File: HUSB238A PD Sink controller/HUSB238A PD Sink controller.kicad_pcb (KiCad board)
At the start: 2 copper layers, 38.1 x 45.7 mm, 74 parts, among them J2 VSET, J4 ISET, J6 I2C, U2 HUSB238A-xxxxx-QN16R

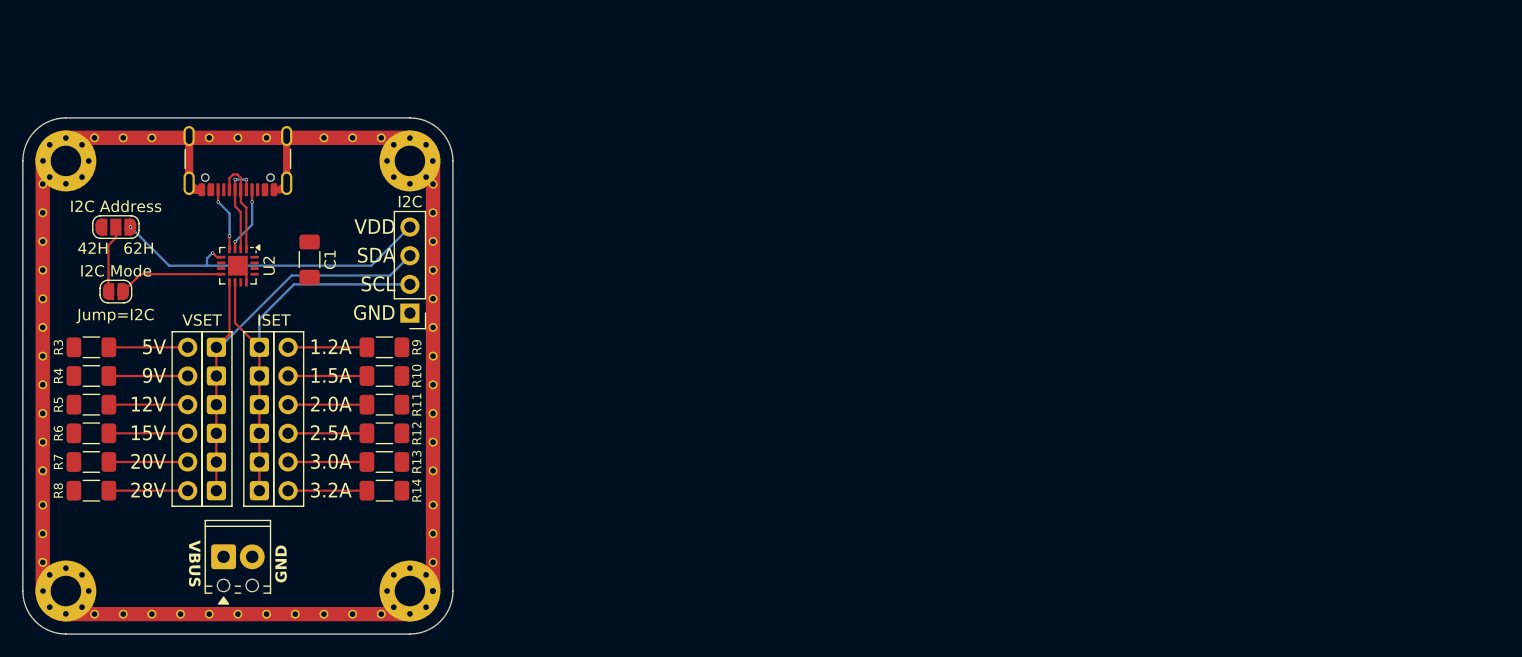
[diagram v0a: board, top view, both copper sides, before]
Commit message: R2.3
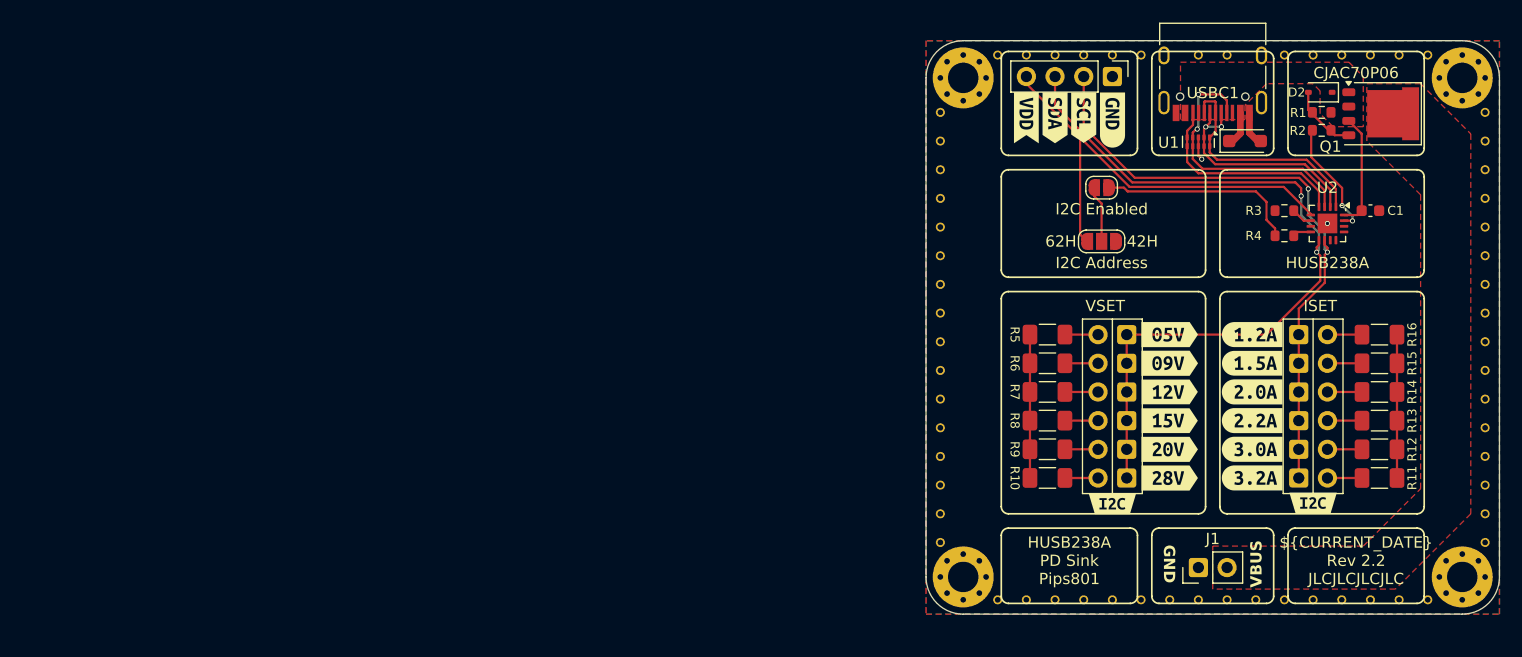
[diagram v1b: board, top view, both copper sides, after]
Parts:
- removed the ? at (94.0, 112.5)
- removed the ? at (84.3, 97.3)
- removed the ? at (88.9, 70.3)
- removed the ? at (118.9, 92.2)
- removed the ? at (118.9, 102.9)
- removed the ? at (99.1, 70.3)
- removed the ? at (84.3, 99.8)
- removed the ? at (118.9, 74.4)
- removed the ? at (84.3, 82.1)
- removed the ? at (84.3, 74.4)
- removed the ? at (114.3, 70.3)
- removed the ? at (118.9, 105.4)
- removed the ? at (118.9, 99.8)
- removed the ? at (84.3, 79.5)
- removed the ? at (118.9, 94.8)
- removed the ? at (84.3, 94.8)
- removed the ? at (84.3, 77.0)
- removed the ? at (106.7, 112.5)
- removed the ? at (91.4, 70.3)
- removed the ? at (84.3, 84.6)
- removed the ? at (118.9, 84.6)
- removed the ? at (104.1, 112.5)
- removed the ? at (118.9, 82.1)
- removed the ? at (84.3, 102.9)
- removed the ? at (114.3, 112.5)
- removed the ? at (118.9, 97.3)
- removed the ? at (84.3, 87.1)
- removed the ? at (104.1, 70.3)
- removed the ? at (111.8, 70.3)
- removed the ? at (84.3, 108.0)
- removed the ? at (99.1, 112.5)
- removed the ? at (96.5, 112.5)
- removed the ? at (84.3, 92.2)
- removed the ? at (101.6, 70.3)
- removed the ? at (118.9, 110.5)
- removed the ? at (94.0, 70.3)
- removed the ? at (118.9, 79.5)
- removed the ? at (118.9, 89.7)
- removed the ? at (118.9, 87.1)
- removed the ? at (88.9, 112.5)
- removed the ? at (91.4, 112.5)
- removed the ? at (84.3, 105.4)
- removed the ? at (109.2, 70.3)
- removed the ? at (101.6, 112.5)
- removed the ? at (84.3, 89.7)
- removed the ? at (109.2, 112.5)
- removed the ? at (118.9, 108.0)
- removed the ? at (118.9, 77.0)
- removed the ? at (111.8, 112.5)
- removed J6: I2C, Connector_PinHeader_2.54mm:PinHeader_1x04_P2.54mm_Vertical
- removed the REF** at (86.4, 110.5)
- removed the REF** at (86.4, 72.4)
- removed the REF** at (116.8, 72.4)
- removed the REF** at (116.8, 110.5)
- added ?: , , F.Cu at (163.8, 78.2)
- added ?: , , F.Cu at (171.4, 111.3)
- added ?: , , F.Cu at (163.8, 83.3)
- added ?: , , F.Cu at (163.8, 70.6)
- added ?: , , F.Cu at (212.1, 75.7)
- added ?: , , F.Cu at (163.8, 73.2)
- added ?: , , F.Cu at (163.8, 106.2)
- added ?: , , F.Cu at (174.0, 63.0)
- added ?: , , F.Cu at (186.7, 111.3)
- added ?: , , F.Cu at (179.1, 63.0)
- added ?: , , F.Cu at (212.1, 93.5)
- added ?: , , F.Cu at (189.2, 63.0)
- added ?: , , F.Cu at (212.1, 106.2)
- added ?: , , F.Cu at (212.1, 90.9)
- added ?: , , F.Cu at (212.1, 85.9)
- added ?: , , F.Cu at (212.1, 68.1)
- added ?: , , F.Cu at (181.6, 111.3)
- added ?: , , F.Cu at (212.1, 83.3)
- added ?: , , F.Cu at (212.1, 70.6)
- added ?: , , F.Cu at (212.1, 88.4)
- added ?: , , F.Cu at (212.1, 73.2)
- added ?: , , F.Cu at (212.1, 103.6)
- added ?: , , F.Cu at (199.4, 63.0)
- added ?: , , F.Cu at (176.5, 63.0)
- added ?: , , F.Cu at (204.5, 63.0)
- added ?: , , F.Cu at (194.3, 63.0)
- added ?: , , F.Cu at (168.9, 111.3)
- added ?: , , F.Cu at (176.5, 111.3)
- added ?: , , F.Cu at (171.4, 63.0)
- added ?: , , F.Cu at (174.0, 111.3)
- added ?: , , F.Cu at (163.8, 85.9)
- added ?: , , F.Cu at (163.8, 88.4)
- added ?: , , F.Cu at (207.0, 63.0)
- added ?: , , F.Cu at (163.8, 90.9)
- added ?: , , F.Cu at (184.2, 111.3)
- added ?: , , F.Cu at (181.6, 63.0)
- added ?: , , F.Cu at (191.8, 111.3)
- added ?: , , F.Cu at (163.8, 101.1)
- added ?: , , F.Cu at (212.1, 96.0)
- added ?: , , F.Cu at (207.0, 111.3)
- added ?: , , F.Cu at (163.8, 103.6)
- added ?: , , F.Cu at (212.1, 98.6)
- added ?: , , F.Cu at (212.1, 78.2)
- added ?: , , F.Cu at (189.2, 111.3)
- added ?: , , F.Cu at (201.9, 111.3)
- added ?: , , F.Cu at (194.3, 111.3)
- added ?: , , F.Cu at (196.8, 63.0)
- added ?: , , F.Cu at (168.9, 63.0)
- added ?: , , F.Cu at (163.8, 80.8)
- added ?: , , F.Cu at (163.8, 68.1)
- added ?: , , F.Cu at (212.1, 80.8)
- added ?: , , F.Cu at (179.1, 111.3)
- added ?: , , F.Cu at (186.7, 63.0)
- added ?: , , F.Cu at (163.8, 75.7)
- added ?: , , F.Cu at (199.4, 111.3)
- added ?: , , F.Cu at (201.9, 63.0)
- added ?: , , F.Cu at (163.8, 96.0)
- added ?: , , F.Cu at (204.5, 111.3)
- added ?: , , F.Cu at (163.8, 98.6)
- added ?: , , F.Cu at (196.8, 111.3)
- added ?: , , F.Cu at (212.1, 101.1)
- added ?: , , F.Cu at (163.8, 93.5)
- added D1: ≥48V TVS Clamp, Diode_SMD:D_SOD-123F, F.Cu at (190.8, 70.6)
- added D2: 15V, Diode_SMD:D_SOD-323, F.Cu at (197.5, 66.3)
- added G***: LOGO, LOGO, B.Cu at (188.0, 87.1)
- added J3: I2C, Connector_PinHeader_2.54mm:PinHeader_1x04_P2.54mm_Vertical, F.Cu at (179.1, 64.9)
- added Q1: CJAC70P06, Package_DFN_QFN:PQFN-8-EP_6x5mm_P1.27mm_Generic, F.Cu at (202.7, 68.2)
- added R1: 100kΩ, Resistor_SMD:R_0603_1608Metric, F.Cu at (197.6, 68.1)
- added R2: 20kΩ, Resistor_SMD:R_0603_1608Metric, F.Cu at (197.6, 69.7)
- added R3: 900kΩ, Resistor_SMD:R_0603_1608Metric, F.Cu at (194.3, 76.8)
- added R4: 900kΩ, Resistor_SMD:R_0603_1608Metric, F.Cu at (194.3, 79.0)
- added REF**: MountingHole_2.7mm_M2.5_Pad_Via, MountingHole:MountingHole_2.7mm_M2.5_Pad_Via, F.Cu at (165.9, 65.0)
- added REF**: MountingHole_2.7mm_M2.5_Pad_Via, MountingHole:MountingHole_2.7mm_M2.5_Pad_Via, F.Cu at (210.1, 65.0)
- added REF**: MountingHole_2.7mm_M2.5_Pad_Via, MountingHole:MountingHole_2.7mm_M2.5_Pad_Via, F.Cu at (210.1, 109.2)
- added REF**: MountingHole_2.7mm_M2.5_Pad_Via, MountingHole:MountingHole_2.7mm_M2.5_Pad_Via, F.Cu at (165.9, 109.2)
- added U1: TPD4E05U06DQA, Package_SON:USON-10_2.5x1.0mm_P0.5mm, F.Cu at (186.7, 70.7)
- added kibuzzard-6951C990: G***, kibuzzard-6951C990, F.Cu at (179.1, 102.8)
- added kibuzzard-6951C990: G***, kibuzzard-6951C990, F.Cu at (196.8, 102.7)
- added kibuzzard-6951CA75: G***, kibuzzard-6951CA75, F.Cu at (184.2, 92.9)
- added kibuzzard-6951CAED: G***, kibuzzard-6951CAED, F.Cu at (184.2, 95.4)
- added kibuzzard-6951CAFD: G***, kibuzzard-6951CAFD, F.Cu at (184.2, 97.9)
- added kibuzzard-6951CB2B: G***, kibuzzard-6951CB2B, F.Cu at (184.2, 100.5)
- added kibuzzard-6951CB42: G***, kibuzzard-6951CB42, F.Cu at (191.5, 87.8)
- added kibuzzard-6951CB4D: G***, kibuzzard-6951CB4D, F.Cu at (191.5, 90.3)
- added kibuzzard-6951CB7E: G***, kibuzzard-6951CB7E, F.Cu at (191.5, 92.9)
- added kibuzzard-6951CEE5: G***, kibuzzard-6951CEE5, F.Cu at (191.5, 95.4)
- added kibuzzard-6951CF0B: G***, kibuzzard-6951CF0B, F.Cu at (191.5, 97.9)
- added kibuzzard-6951CF1D: G***, kibuzzard-6951CF1D, F.Cu at (191.5, 100.5)
- added kibuzzard-6951CF39: G***, kibuzzard-6951CF39, F.Cu at (184.2, 87.8)
- added kibuzzard-6951CF4B: G***, kibuzzard-6951CF4B, F.Cu at (184.2, 90.3)
- added kibuzzard-6951D5A7: G***, kibuzzard-6951D5A7, F.Cu at (179.1, 68.8)
- added kibuzzard-6951D5B1: G***, kibuzzard-6951D5B1, F.Cu at (176.5, 68.6)
- added kibuzzard-6951D5BC: G***, kibuzzard-6951D5BC, F.Cu at (174.0, 68.6)
- added kibuzzard-6951D5C7: G***, kibuzzard-6951D5C7, F.Cu at (171.4, 68.6)
- C1: footprint Capacitor_SMD:C_1206_3216Metric_Pad1.33x1.80mm_HandSolder -> Capacitor_SMD:C_0603_1608Metric
- J1: renamed from REF**; value TerminalBlock_Phoenix_MPT-0,5-2-2.54_1x02_P2.54mm_Horizontal -> VBUS; footprint TerminalBlock_Phoenix:TerminalBlock_Phoenix_MPT-0,5-2-2.54_1x02_P2.54mm_Horizontal -> Connector_PinHeader_2.54mm:PinHeader_1x02_P2.54mm_Vertical
- JP1: renamed from JP3; value I2C Mode -> I2C Enabled
- U2: value HUSB238A-xxxxx-QN16R -> HUSB238A
- USBC1: footprint Connector_USB:USB_C_Receptacle_GCT_USB4105-xx-A_16P_TopMnt_Horizontal -> Connector_USB:USB_C_Receptacle_HRO_TYPE-C-31-M-12
- moved U2 96.6 mm to (198.1, 77.9)
- moved C1 94.1 mm to (201.9, 76.8), turned to 0 degrees
- moved J4 92.1 mm to (195.6, 87.8)
- moved R11 88.2 mm to (202.7, 100.5)
- moved R12 88.2 mm to (202.7, 97.9)
- moved R13 88.2 mm to (202.7, 95.4)
- moved R14 88.2 mm to (202.7, 92.9)
- moved R15 88.2 mm to (202.7, 90.3)
- moved R16 88.2 mm to (202.7, 87.8)
- moved JP1 87.8 mm to (178.1, 74.8)
- moved JP2 87.3 mm to (178.1, 79.5)
- moved USBC1 86.7 mm to (188.0, 64.1)
- moved J1 86.4 mm to (186.7, 108.4), turned to 90 degrees
- moved R10 84.7 mm to (173.3, 100.5)
- moved R5 84.7 mm to (173.3, 87.8)
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- renumbered R8 to R10, R14 to R11, R13 to R12, R12 to R13, R11 to R14, R10 to R15, R9 to R16, R3 to R5, R4 to R6, R5 to R7, R6 to R8, R7 to R9
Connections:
- J1 pad 1: (no net) -> GND
- J1 pad 2: (no net) -> VBUS_OUT
- JP1 pad 2: GPIO/I2C -> Net-(JP1-B)
- JP2 pad 1: GND -> VDD
- JP2 pad 3: VDD -> GND
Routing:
- net VSET/SDA: track 39.4 -> 68.8 mm, vias 0 -> 2
- net Net-(JP1-B): track 0.00 -> 18.2 mm
- net ISET/SCL: track 36.5 -> 54.6 mm, vias 0 -> 2
- net CC1: track 5.88 -> 24.0 mm
- net GND: track 12.8 -> 30.5 mm, vias 0 -> 2
- net VBUS: track 0.00 -> 13.2 mm
- net CC2: track 5.68 -> 18.7 mm, vias 2 -> 0
- net D-: track 8.28 -> 20.4 mm
- net D+: track 8.81 -> 20.8 mm
- net GATE: track 0.00 -> 10.3 mm, vias 0 -> 2
- net VDD: track 29.9 -> 39.5 mm, vias 2 -> 0
- net GPIO/I2C: track 9.32 -> 1.65 mm
- net Net-(D2-A): track 0.00 -> 6.23 mm
- net /9V: track 6.98 -> 2.93 mm
- net /15V: track 6.98 -> 2.93 mm
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- added copper zone on B.Cu, net GND
- added copper zone on F.Cu, net GND
- added copper zone on F.Cu, net VBUS
- added copper zone on F.Cu, net VBUS_OUT
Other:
- board size 38.1 x 45.7 mm -> 50.8 x 50.8 mm
- board text added: "${COMMENT1} PD Sink Pips801"
- board text added: "${CURRENT_DATE} ${REVISION} JLCJLCJLCJLC"
- board text removed: "1.2A"
- board text removed: "1.5A"
- board text removed: "12V"
- board text removed: "15V"
- board text removed: "2.0A"
- board text removed: "2.5A"
- board text removed: "20V"
- board text removed: "28V"
- board text removed: "3.0A"
- board text removed: "3.2A"
- board text removed: "5V"
- board text removed: "9V"
- board text removed: "Jump=I2C"
- board text removed: "SCL"
- board text removed: "SDA"
- board text removed: "VDD"
